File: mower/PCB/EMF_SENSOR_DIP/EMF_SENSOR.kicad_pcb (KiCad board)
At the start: 2 copper layers, 40 x 40 mm, 15 parts, among them J1 Conn_01x03_Pin, U1 LM358

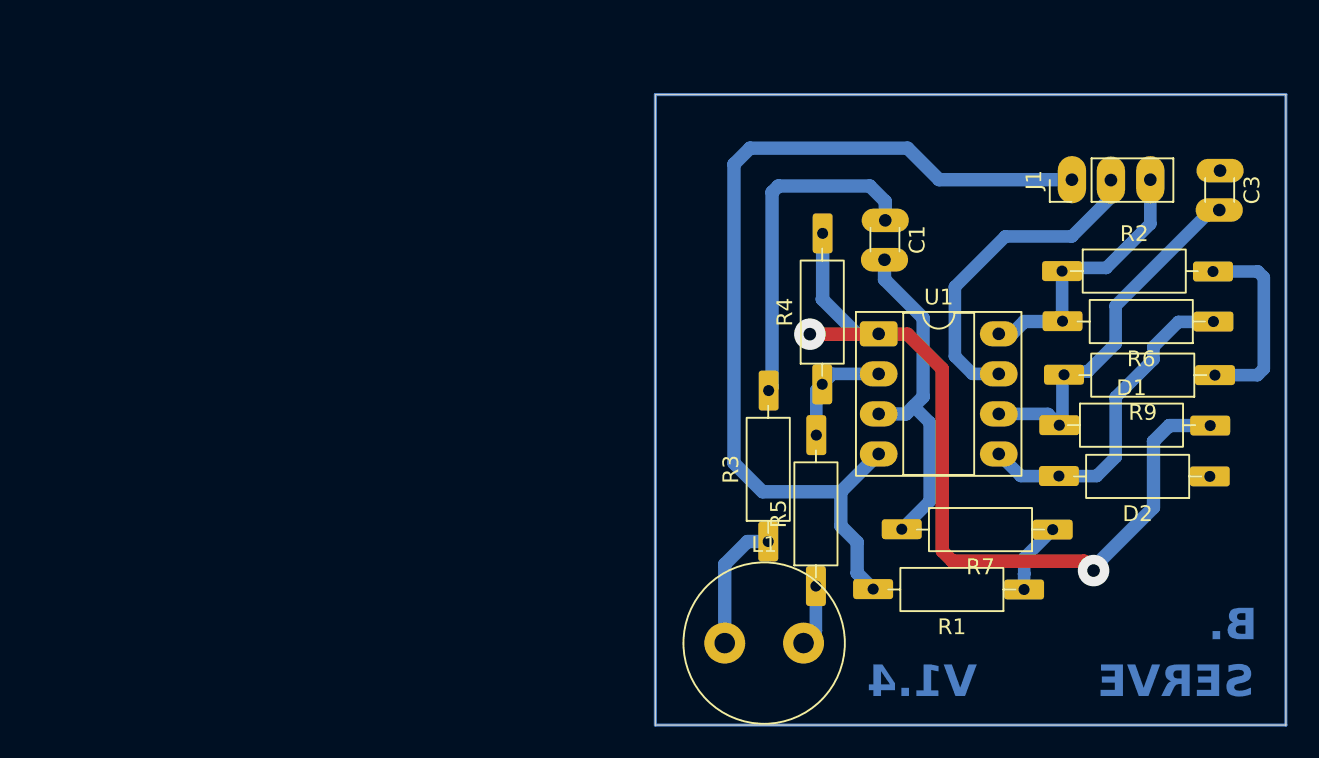
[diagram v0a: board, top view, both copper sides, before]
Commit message: .
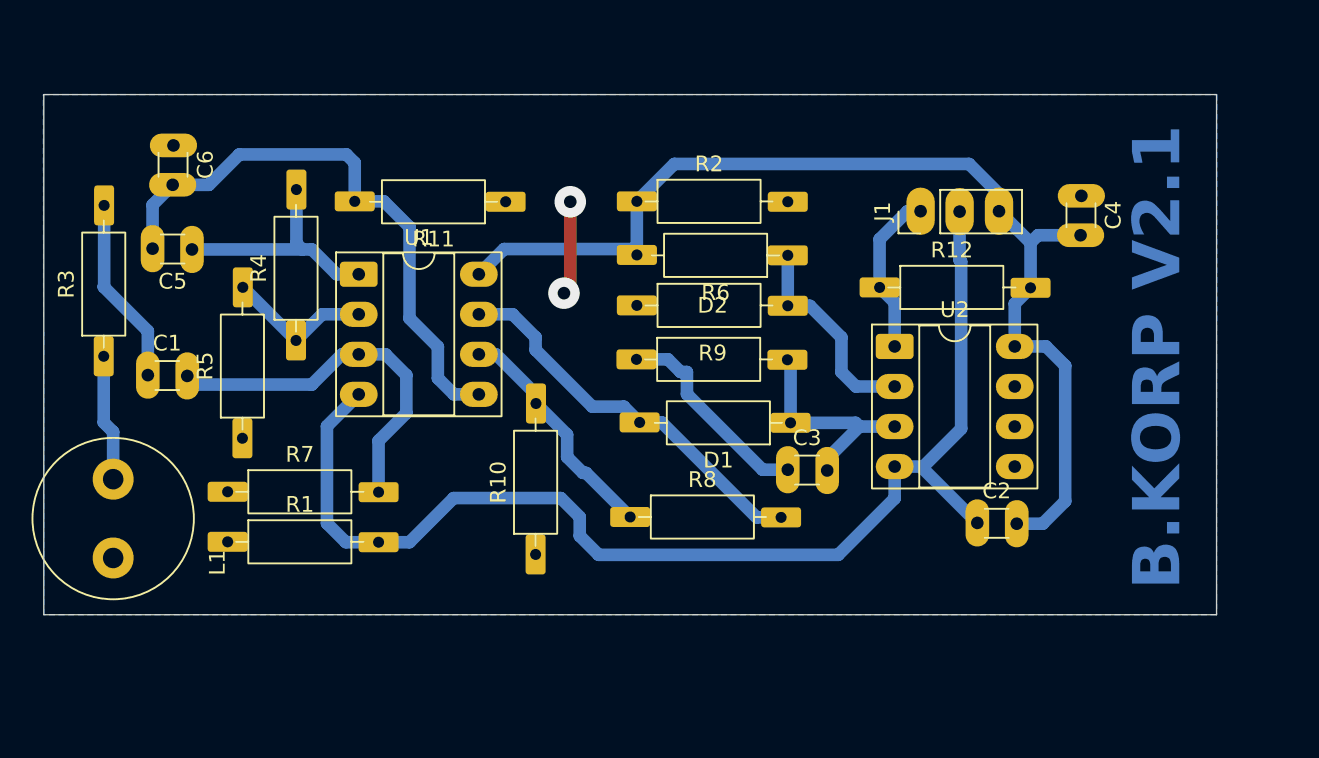
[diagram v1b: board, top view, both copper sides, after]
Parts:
- added C2: 10uF, IMRANS_LIBRARY:C_Disc_D3.0mm_W1.6mm_P2.50mm, F.Cu at (158.4, 65.2)
- added C4: 10uF, IMRANS_LIBRARY:C_Disc_D3.0mm_W1.6mm_P2.50mm, F.Cu at (165.0, 44.4)
- added C5: 1nF, IMRANS_LIBRARY:C_Disc_D3.0mm_W1.6mm_P2.50mm, F.Cu at (108.6, 47.8)
- added C6: 0.01uF, IMRANS_LIBRARY:C_Disc_D3.0mm_W1.6mm_P2.50mm, F.Cu at (107.4, 41.2)
- added R10: 10K, IMRANS_LIBRARY:R_Axial_DIN0207_L6.3mm_D2.5mm_P10.16mm_Horizontal_2, F.Cu at (130.4, 67.7)
- added R11: 10K, IMRANS_LIBRARY:R_Axial_DIN0207_L6.3mm_D2.5mm_P10.16mm_Horizontal_2, F.Cu at (129.0, 44.8)
- added R12: 100K, IMRANS_LIBRARY:R_Axial_DIN0207_L6.3mm_D2.5mm_P10.16mm_Horizontal_2, F.Cu at (151.7, 50.2)
- added R8: 1M, IMRANS_LIBRARY:R_Axial_DIN0207_L6.3mm_D2.5mm_P10.16mm_Horizontal_2, F.Cu at (135.9, 64.8)
- added U2: LM393, Package_DIP:DIP-8_W7.62mm_Socket_LongPads, F.Cu at (153.2, 54.0)
- D2: value D -> 1N5819
- R7: value 1K -> 10K
- moved R7 53.4 mm to (110.4, 63.2), turned to 0 degrees
- moved R1 51.6 mm to (110.4, 66.4), turned to 0 degrees
- moved C1 47.8 mm to (105.8, 55.8), turned to 0 degrees
- moved R3 43.8 mm to (103.0, 55.1)
- moved L1 40.2 mm to (103.6, 62.4), turned to -90 degrees
- moved D2 38.9 mm to (136.3, 51.4), turned to 0 degrees
- moved R9 37.7 mm to (136.3, 54.8), turned to 0 degrees
- moved R5 37.6 mm to (111.8, 60.3)
- moved R4 33.5 mm to (115.2, 54.1)
- moved C3 33.4 mm to (146.4, 61.8), turned to 0 degrees
- moved U1 33.2 mm to (119.2, 49.4)
- moved R2 27.3 mm to (136.3, 44.8)
- moved R6 27.3 mm to (146.9, 48.2)
- moved D1 16.1 mm to (147.1, 58.8), turned to 180 degrees
- moved J1 9.81 mm to (154.8, 45.4)
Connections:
- J1 pad 1: GND -> Net-(J1-Pin_1)
- J1 pad 2: Net-(J1-Pin_2) -> GND
- R4 pad 2: Net-(D1-A) -> Net-(C5-Pad1)
- U1 pad 1: Net-(D1-A) -> Net-(C5-Pad1)
- U1 pad 5: Net-(D2-A) -> Net-(U1B-+)
- U1 pad 6: Net-(D1-K) -> Net-(U1B--)
- U1 pad 7: Net-(J1-Pin_2) -> Net-(D1-A)
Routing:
- net VCC: track 17.7 -> 69.3 mm
- net Net-(U1B-+): track 0.00 -> 37.1 mm
- net Net-(D1-A): track 57.8 -> 25.0 mm, vias 2 -> 0
- net Net-(J1-Pin_2): track 21.0 -> 0.00 mm
- net GND: track 59.9 -> 76.4 mm
- net Net-(U1B--): track 0.00 -> 15.9 mm
- net Net-(C5-Pad1): track 0.00 -> 15.2 mm
- net Net-(J1-Pin_1): track 0.00 -> 10.5 mm
- net Net-(C1-Pad1): track 21.6 -> 11.9 mm
- net Net-(D1-K): track 23.2 -> 14.2 mm
- net Net-(D2-A): track 20.9 -> 13.4 mm
- net Net-(U1A--): track 7.23 -> 9.44 mm
- net Net-(U1A-+): track 21.9 -> 23.6 mm
- net GNDREF: track 20.9 -> 19.3 mm, vias 0 -> 2
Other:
- board size 40 x 40 mm -> 74.4 x 33 mm
- board text added: "B.KORP V2.1"
- board text removed: "B."
- board text removed: "SERVE"
- board text removed: "V1.4"

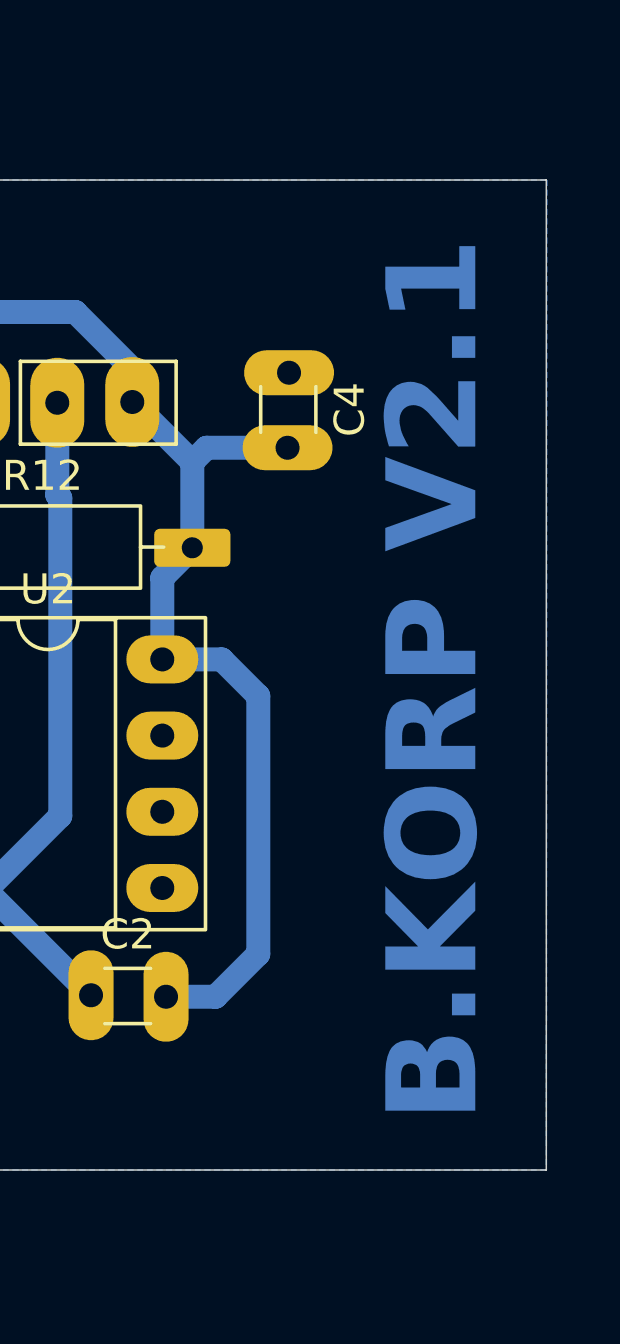
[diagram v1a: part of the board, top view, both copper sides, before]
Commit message: .
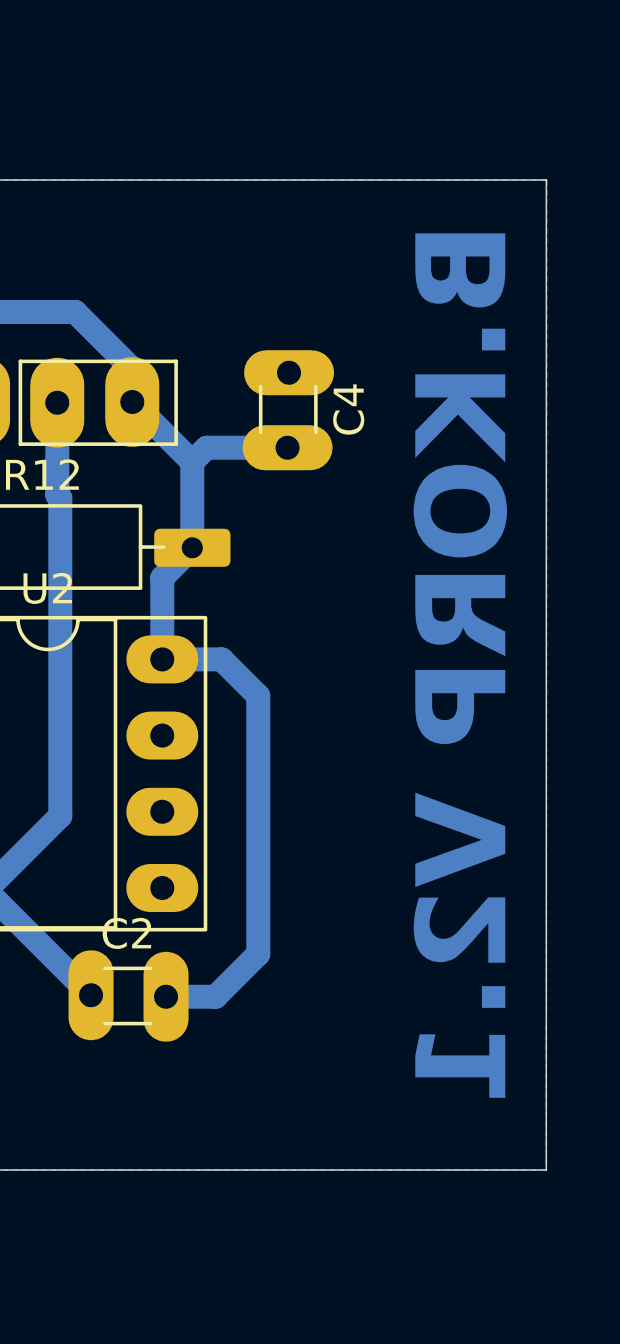
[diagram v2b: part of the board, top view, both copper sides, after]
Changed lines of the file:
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@@
 	)
 	(gr_text "B.KORP V2.1"
-		(at 171.6 69.4 90)
+		(at 172.6 39.4 90)
 		(layer "B.Cu" knockout)
 		(effects
@@
 				(bold yes)
 			)
-			(justify left bottom)
+			(justify left bottom mirror)
 		)
 	)
